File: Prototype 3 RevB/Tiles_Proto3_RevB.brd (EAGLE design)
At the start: 40 x 40 mm, 62 parts, among them Q1 DMG3415U-7, U2 MF-DSC-SOT233-MMBT3904, X1 32.768

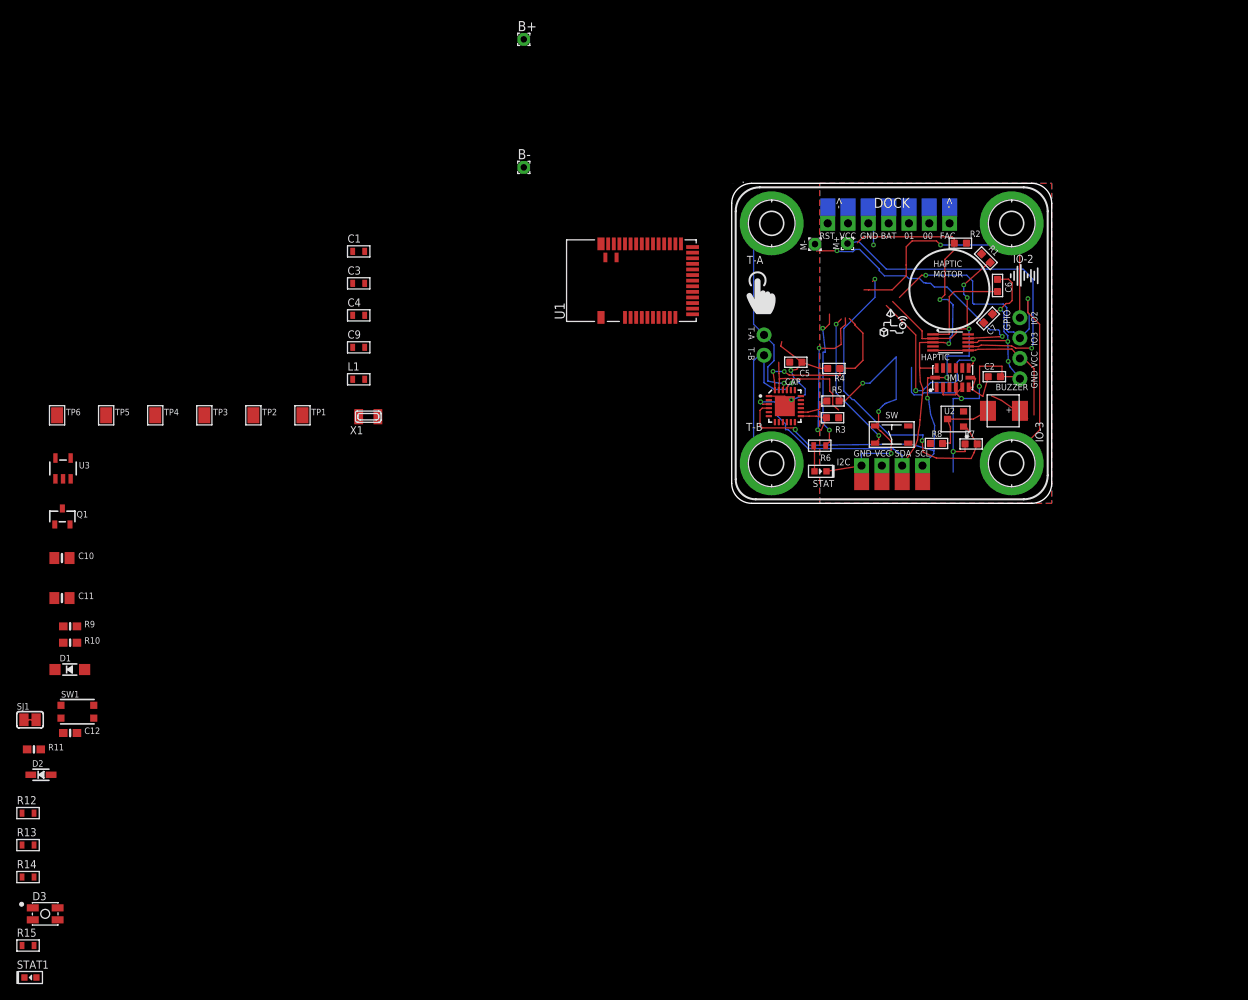
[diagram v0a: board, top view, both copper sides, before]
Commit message: finished placing proto3revB
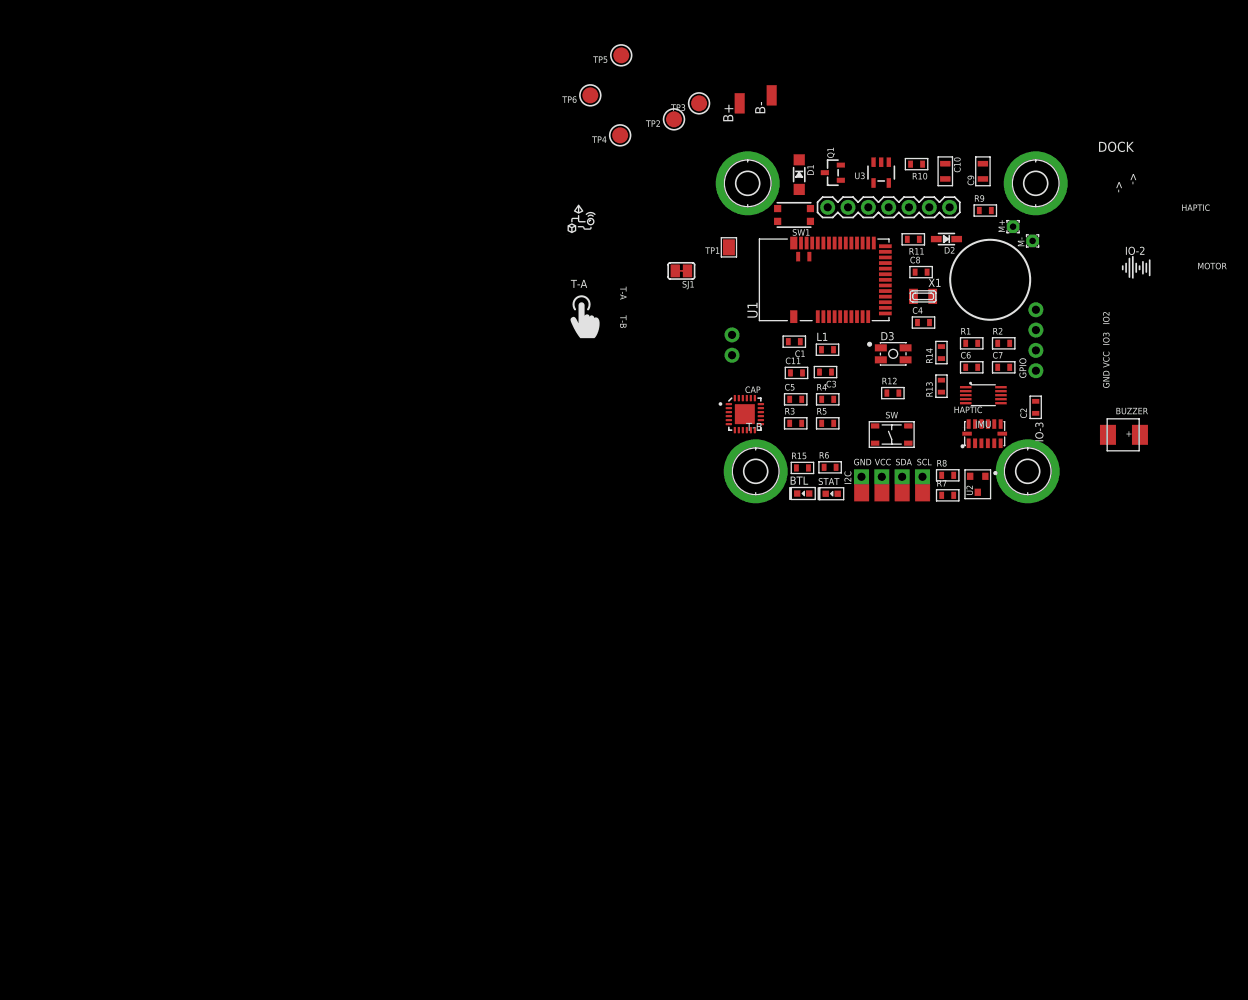
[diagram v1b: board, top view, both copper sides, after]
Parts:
- removed C12: 0.1uF, microbuilder2:0603-NO
- removed STAT1: MF-LED-0603-RED, MF_LEDs:LED0603
- added BTL: MF-LED-0603-RED, MF_LEDs:LED0603
- added C8: (no value), MF_Passives:C0603
- B+, B-: device wirepad:1,6/0,8 -> wirepad:SMD1,27-2,54
- C1: value 1uF -> (none)
- C10: value 10µF -> (none); device microbuilder2:0805-NO -> MF_Passives:C0805
- C11: value 10µF -> (none); device microbuilder2:0805-NO -> MF_Passives:C0603
- C2: value 100nf -> (none); device Seeed-OPL-Capacitor:C0603 -> MF_Passives:C0603
- C3: value 10uF -> (none)
- C4: value 22pF -> (none)
- C5: value 10uf -> (none); device Seeed-OPL-Capacitor:C0603 -> MF_Passives:C0603
- C6, C7: value 1uf -> (none); device Seeed-OPL-Capacitor:C0603 -> MF_Passives:C0603
- C9: value 22pF -> (none); device MF_Passives:C0603 -> MF_Passives:C0805
- J1: device tiles:1X07_SQUAREPADS_BOTTOM -> SparkFun-Connectors:1X07
- R1, R2, R3, R4, R7: value 10K 1/10W -> (none); device Seeed-OPL-Resistor:R0603 -> MF_Passives:R0603
- R10, R9: value 100K -> (none); device microbuilder2:0603-NO -> MF_Passives:R0603
- R11: value 10K -> (none); device microbuilder2:0603-NO -> MF_Passives:R0603
- R12, R13, R14, R15, R6: value 330 -> (none)
- R5: value 100K 1/10W -> (none); device Seeed-OPL-Resistor:R0603 -> MF_Passives:R0603
- R8: value 1K 1/10W -> (none); device Seeed-OPL-Resistor:R0603 -> MF_Passives:R0603
- TP2, TP3, TP4, TP5, TP6: device microbuilder2:PAD-1.5X2.0 -> microbuilder2:TESTPOINT_ROUND_2MM
- moved R14 131.7 mm to (26.2, -21.2), turned to 90 degrees
- moved D2 131.5 mm to (26.8, -6.97), turned to 180 degrees
- moved R13 127.8 mm to (26.2, -25.4), turned to 90 degrees
- moved R11 127.1 mm to (22.7, -7.00), turned to 180 degrees
- moved D3 127.0 mm to (20.2, -21.3)
- moved R9 125.7 mm to (31.7, -3.40)
- moved R10 121.5 mm to (23.1, 2.40), turned to 180 degrees
- moved C10 120.5 mm to (26.7, 1.50), turned to 270 degrees
- moved R12 120.2 mm to (20.1, -26.2)
- moved R15 113.7 mm to (8.84, -35.6)
- moved D1 110.2 mm to (8.44, 1.09), turned to 270 degrees
- moved SW1 109.0 mm to (7.79, -3.95), turned to 180 degrees
- moved U3 108.8 mm to (18.7, 1.34), turned to 180 degrees
- moved Q1 105.5 mm to (12.6, 1.33), turned to 90 degrees
- moved SJ1 98.9 mm to (-6.29, -10.9), turned to 180 degrees
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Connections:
- net 3.3V: now also C2.P$1, C5.P$1, C7.P$1, C9.P$1, R1.P$1, R11.P$2, R2.P$1, R3.P$1, R8.P$1; no longer C10.1, C2.1, C5.1, C7.2, R1.1, R11.1, R2.2, R3.2, R8.2
- net BUZZER: now also R7.P$2; no longer R7.2
- net CAP-INT: now also R3.P$2; no longer R3.1
- net CAP-RES: now also R4.P$1; no longer R4.2
- net DTR: now also C11.P$1; no longer C12.1
- net GND: now also BTL.CATHODE, C10.P$2, C2.P$2, C5.P$2, C6.P$2, C7.P$2, C8.P$2, R4.P$2, R5.P$2, R7.P$1, R9.P$2; no longer C10.2, C11.2, C2.2, C5.2, C6.1, C7.1, R4.1, R5.1, R7.1, R9.2, STAT1.CATHODE
- net N$10: now also R10.P$2; no longer R10.2
- net N$12: now also C8.P$1; no longer C9.P$1
- net N$13: now also C10.P$1, R10.P$1; no longer C11.1, R10.1
- net N$18: now also BTL.ANODE; no longer STAT1.ANODE
- net N$20: now also C11.P$2; no longer C12.2
- net N$3: now also R5.P$1; no longer R5.2
- net N$4: now also R8.P$2; no longer R8.1
- net N$5: now also C6.P$1; no longer C6.2
- net RESET: now also R11.P$1; no longer R11.2
- net SCL: now also R1.P$2; no longer R1.2
- net SDA: now also R2.P$2; no longer R2.1
- net VBUS: now also R9.P$1; no longer R9.1
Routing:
- net GND: track 120.2 -> 0.00 mm, vias 12 -> 0
- net SDA: track 73.7 -> 0.00 mm, vias 3 -> 0
- net SCL: track 72.4 -> 0.00 mm, vias 6 -> 0
- net IO-3: track 50.7 -> 0.00 mm, vias 2 -> 0
- net 3.3V: track 47.9 -> 0.00 mm
- net N$8: track 42.1 -> 0.00 mm, vias 1 -> 0
- net BUZZER: track 41.4 -> 0.00 mm, vias 2 -> 0
- net IO-2: track 37.5 -> 0.00 mm, vias 1 -> 0
- net N$7: track 33.4 -> 0.00 mm, vias 2 -> 0
- net CAP-A: track 27.4 -> 0.00 mm, vias 1 -> 0
- net CAP-B: track 25.2 -> 0.00 mm, vias 1 -> 0
- net IMU-INT: track 23.7 -> 0.00 mm, vias 2 -> 0
- net CAP-INT: track 22.1 -> 0.00 mm, vias 2 -> 0
- net CAP-RES: track 21.0 -> 0.00 mm, vias 2 -> 0
- net BTN: track 18.2 -> 0.00 mm, vias 2 -> 0
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- removed copper zone on layer 1, net GND
- removed copper zone on layer 16, net GND
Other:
- board outline removed
- board text removed: "/Users/Simone/Downloads/digi.bmp"
- board text removed: "00"
- board text removed: "01"
- board text removed: "BAT"
- board text removed: "FAC"
- board text removed: "RST"

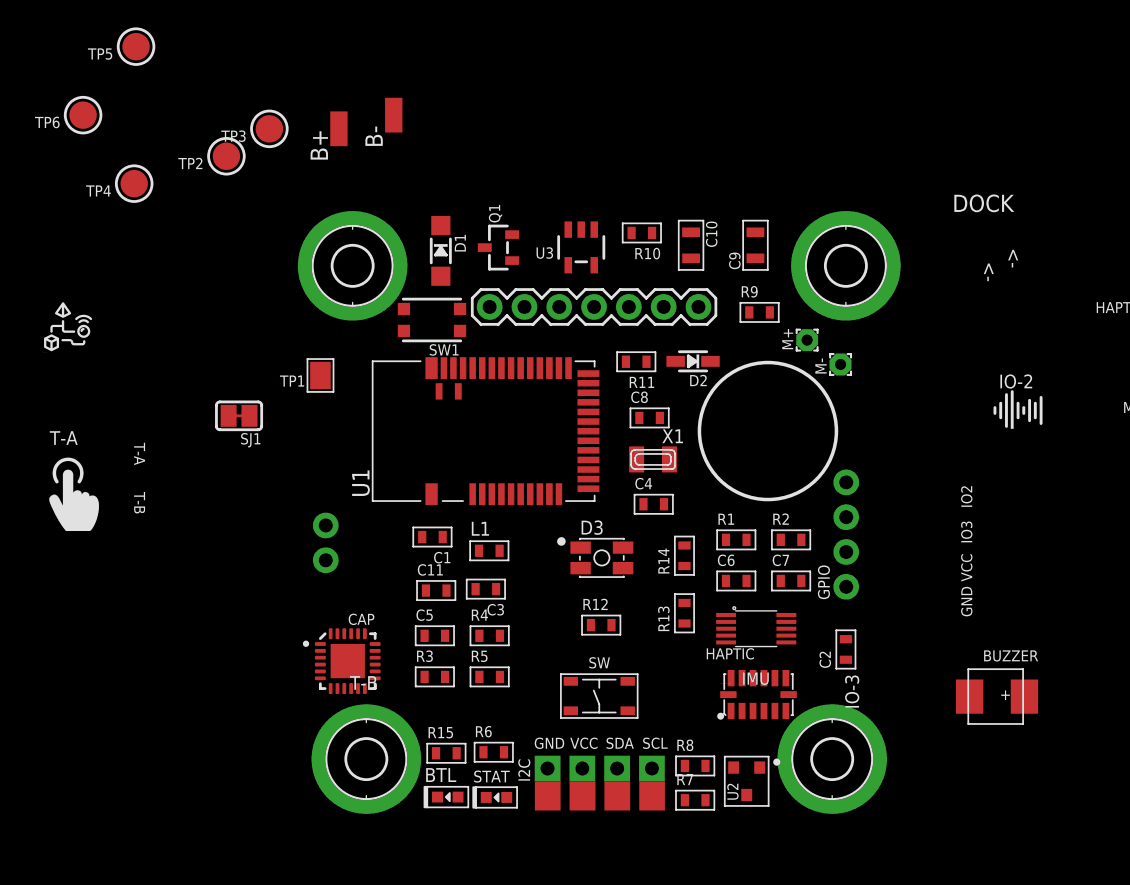
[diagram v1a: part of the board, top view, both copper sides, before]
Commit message: partial routing
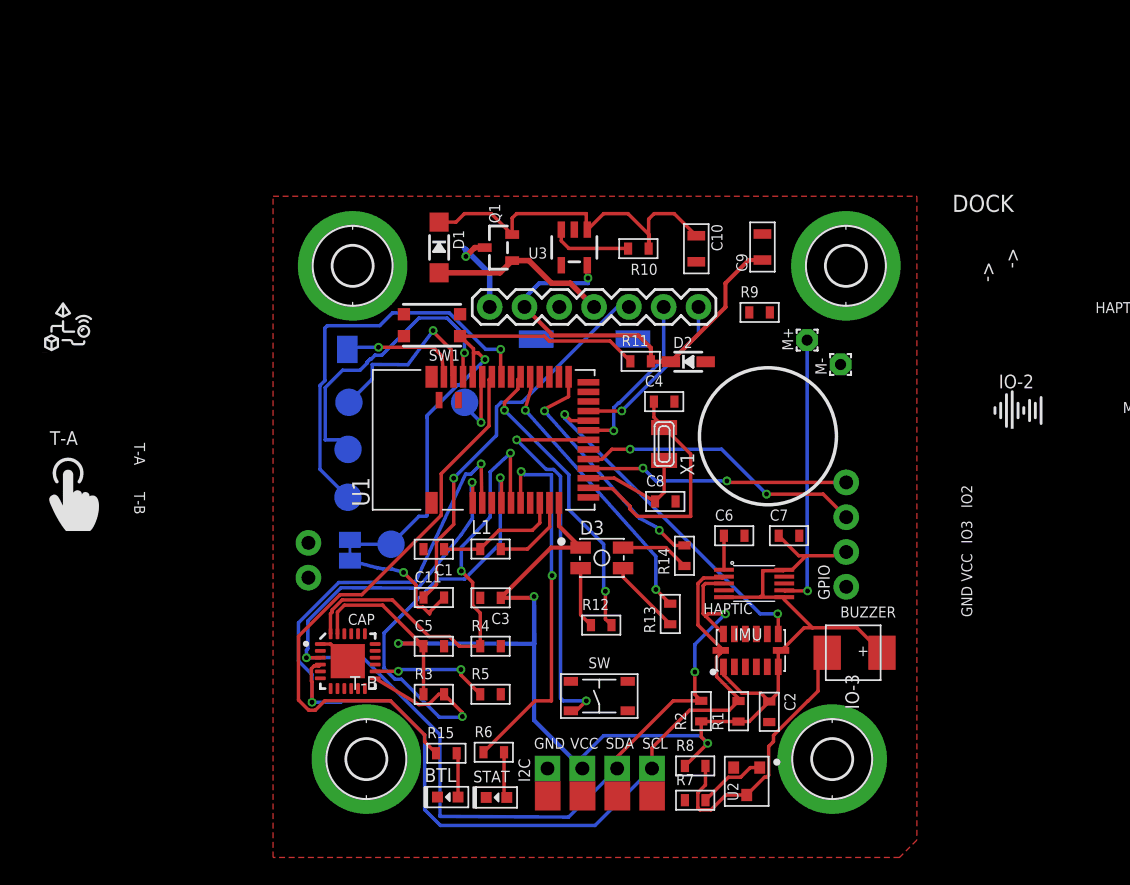
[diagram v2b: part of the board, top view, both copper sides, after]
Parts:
- removed TP1: (no value), microbuilder2:PAD-1.5X2.0
- removed TP2, TP3, TP4, TP5, TP6: (no value), microbuilder2:TESTPOINT_ROUND_2MM
- added DFU, RST, SWCLK, SWDIO, SWO: (no value), microbuilder2:TESTPOINT_ROUND_2MM
- added FRST: (no value), microbuilder2:PAD-1.5X2.0
- moved B- 23.9 mm to (22.5, -5.34), flipped to the bottom, turned to 270 degrees
- moved B+ 21.0 mm to (15.4, -5.35), flipped to the bottom, turned to 270 degrees
- moved R2 14.1 mm to (27.4, -32.5), turned to 90 degrees
- moved SJ1 12.7 mm to (1.80, -20.8), flipped to the bottom, turned to 270 degrees
- moved R1 12.5 mm to (30.2, -32.5), turned to 90 degrees
- moved BUZZER 10.9 mm to (38.8, -28.5)
- moved C4 7.53 mm to (24.7, -9.91)
- moved C2 7.21 mm to (32.4, -32.5), turned to 270 degrees
- moved C8 6.20 mm to (24.8, -17.2)
- moved HAPTIC 3.31 mm to (31.0, -23.2)
- moved C6 3.31 mm to (29.8, -19.7)
- moved C7 3.31 mm to (33.8, -19.7)
- moved IMU 3.28 mm to (31.1, -28.1)
- moved TOUCH 1.80 mm to (-1.23, -20.2)
- moved X1 1.39 mm to (24.7, -13.0), turned to 90 degrees
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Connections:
- net DFU: now also DFU.P$1; no longer TP5.P$1
- net FRST: now also FRST.P$1; no longer TP1.P$1
- net RESET: now also RST.P$1; no longer TP4.P$1
- net SWCLK: now also SWCLK.P$1; no longer TP3.P$1
- net SWDIO: now also SWDIO.P$1; no longer TP2.P$1
- net SWO: now also SWO.P$1; no longer TP6.P$1
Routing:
- net 3.3V: track 0.00 -> 143.8 mm, vias 0 -> 4
- net SCL: track 0.00 -> 87.1 mm, vias 0 -> 2
- net SDA: track 0.00 -> 79.3 mm, vias 0 -> 4
- net BT_LED: track 0.00 -> 42.9 mm
- net RESET: track 0.00 -> 37.5 mm, vias 0 -> 1
- net CAP-INT: track 0.00 -> 35.7 mm, vias 0 -> 2
- net CAP-RES: track 0.00 -> 34.1 mm, vias 0 -> 2
- net SWO: track 0.00 -> 29.8 mm, vias 0 -> 1
- net BTN: track 0.00 -> 29.1 mm, vias 0 -> 2
- net DTR: track 0.00 -> 28.8 mm, vias 0 -> 1
- net STATLED: track 0.00 -> 27.7 mm, vias 0 -> 2
- net N$13: track 0.00 -> 27.3 mm
- net IMU-INT: track 0.00 -> 25.1 mm, vias 0 -> 2
- net LED_R: track 0.00 -> 21.8 mm, vias 0 -> 2
- net SWCLK: track 0.00 -> 21.7 mm, vias 0 -> 1
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- added copper zone on layer 1, net GND
